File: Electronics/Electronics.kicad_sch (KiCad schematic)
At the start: 0 parts

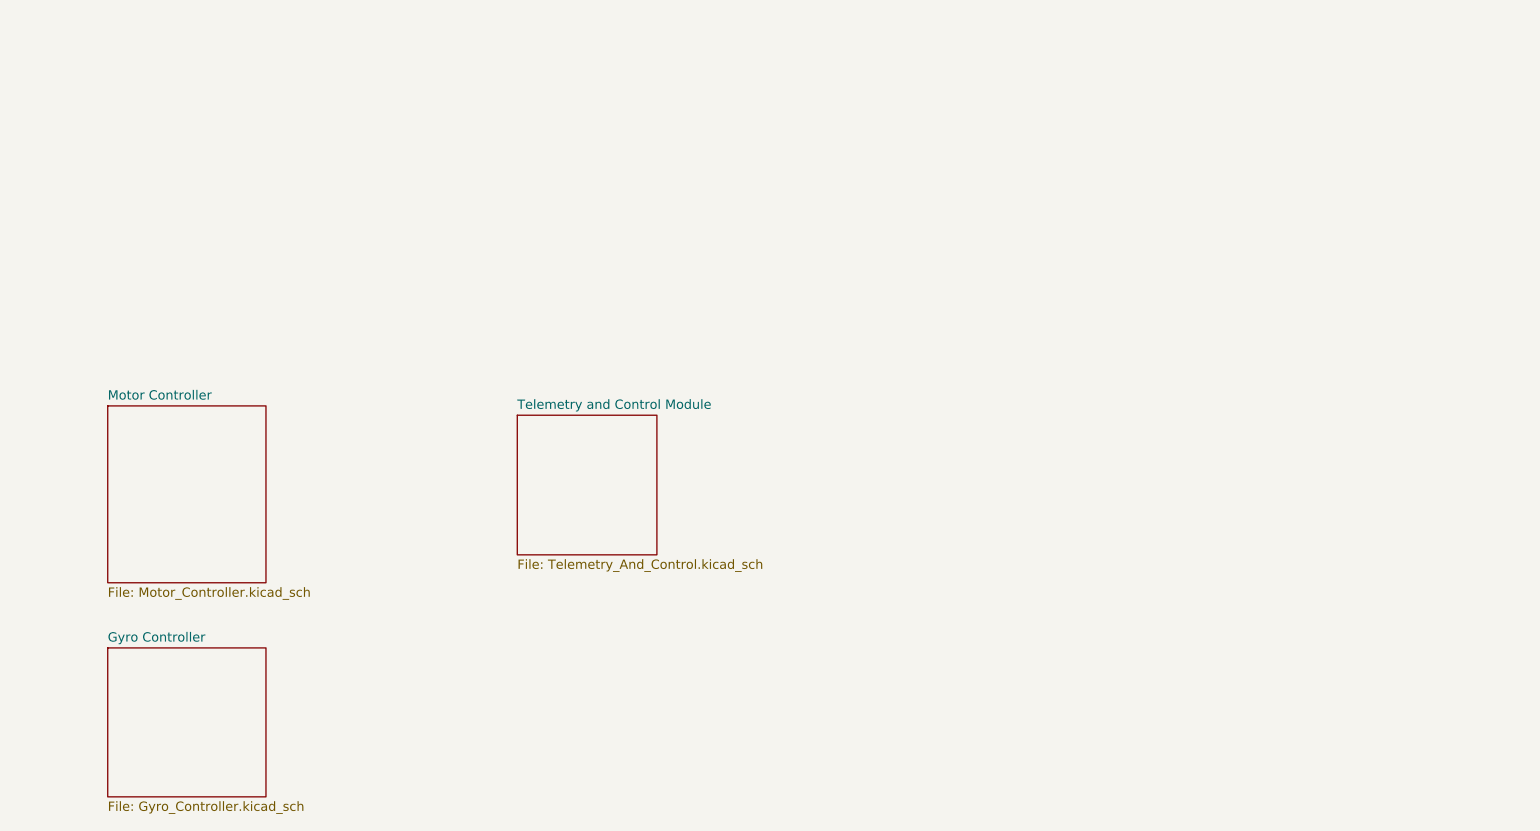
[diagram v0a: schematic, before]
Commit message: power + usb
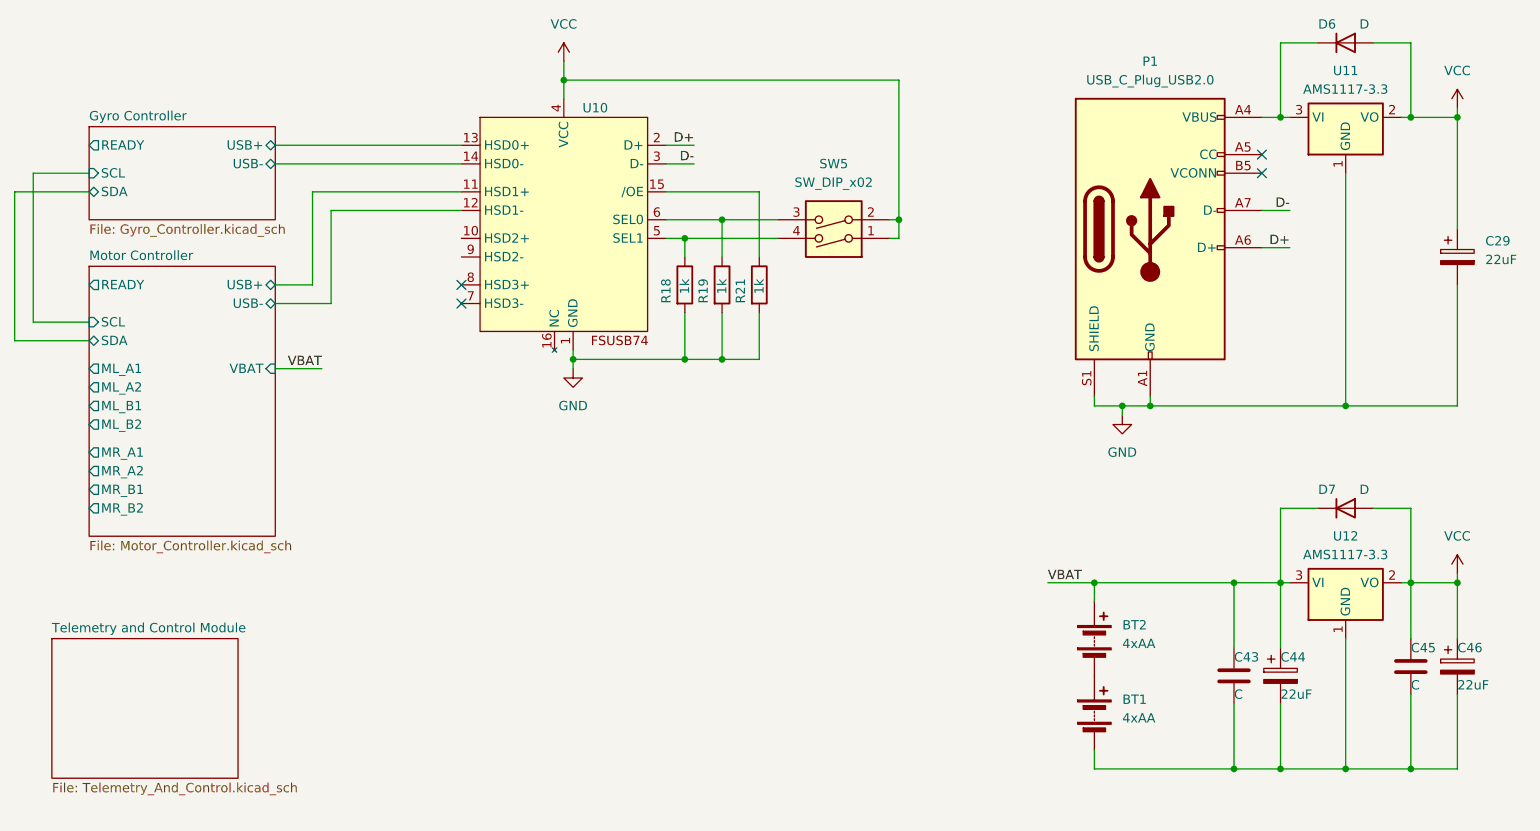
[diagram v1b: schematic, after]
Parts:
- added BT1, BT2: 4xAA, symbol Device:Battery
- added C29, C44, C46: 22uF, symbol Device:C_Polarized
- added C43, C45: C, symbol Device:C
- added D6, D7: D, symbol Device:D
- added P1: USB_C_Plug_USB2.0, symbol Connector:USB_C_Plug_USB2.0
- added R18, R19, R21: 1k, symbol Device:R
- added SW5: SW_DIP_x02, symbol Switch:SW_DIP_x02
- added U10: ~, Package_DFN_QFN:QFN-16-1EP_3x3mm_P0.5mm_EP1.7x1.7mm, symbol FSUSB74:FSUSB74
- added U11, U12: AMS1117-3.3, Package_TO_SOT_SMD:SOT-223-3_TabPin2, symbol Regulator_Linear:AMS1117-3.3
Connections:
- new net: BT1.2 (-), C43.2, C44.2, C45.2, C46.2, U12.1 (GND)
- new net: R19.1, SW5.3, U10.6 (SEL0)
- new net: R21.1, U10.15 (/OE)
- new net: R18.1, SW5.4, U10.5 (SEL1)
- new net: D6.1 (K), P1.A4 (VBUS), P1.A9 (VBUS), P1.B4 (VBUS), P1.B9 (VBUS), U11.3 (VI)
- new net: BT1.1 (+), BT2.2 (-)
- new net D+: P1.A6 (D+), U10.2 (D+)
- new net D-: P1.A7 (D-), U10.3 (D-)
- new net GND: C29.2, P1.A1 (GND), P1.A12 (GND), P1.B1 (GND), P1.B12 (GND), P1.S1 (SHIELD), R18.2, R19.2, R21.2, U10.1 (GND), U11.1 (GND)
- new net Gyro Controller/USB+: U10.13 (HSD0+)
- new net Gyro Controller/USB-: U10.14 (HSD0-)
- new net Motor Controller/USB+: U10.11 (HSD1+)
- new net Motor Controller/USB-: U10.12 (HSD1-)
- new net VBAT: BT2.1 (+), C43.1, C44.1, D7.1 (K), U12.3 (VI)
- new net VCC: C29.1, C45.1, C46.1, D6.2 (A), D7.2 (A), SW5.1, SW5.2, U10.4 (VCC), U11.2 (VO), U12.2 (VO)
- no-connect marks 0 -> 4
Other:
- sheet Gyro Controller ports: added READY, SCL, SDA, USB+, USB-; removed none
- sheet Motor Controller ports: added ML_A1, ML_A2, ML_B1, ML_B2, MR_A1, MR_A2, MR_B1, MR_B2, READY, SCL, SDA, USB+, USB-, VBAT; removed none
